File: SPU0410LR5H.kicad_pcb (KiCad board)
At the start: 2 copper layers, 23 x 12.5 mm, 17 parts, among them J1 Conn_01x04_Pin, U1 MCP6002-xSN, U2 SPU0410LR5H-QB

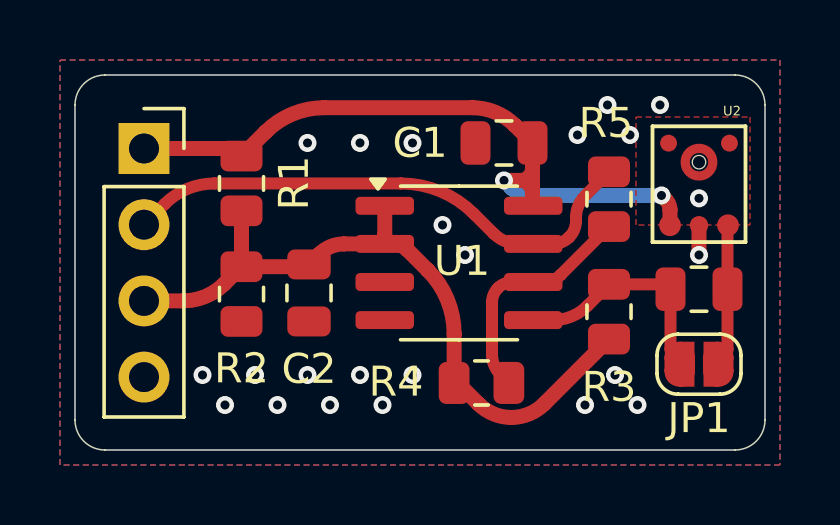
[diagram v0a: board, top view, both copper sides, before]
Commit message: update silkscreen
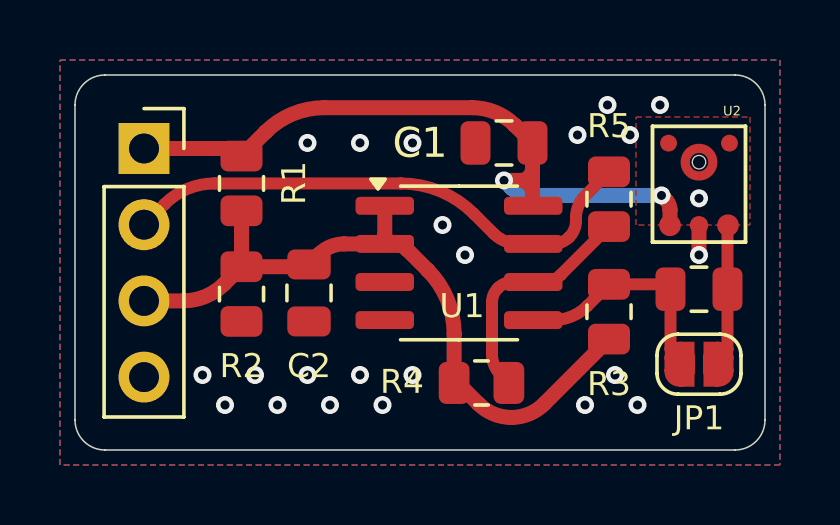
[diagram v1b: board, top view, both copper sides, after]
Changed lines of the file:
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@@
 			(outputformat 1)
 			(mirror no)
-			(drillshape 1)
+			(drillshape 0)
 			(scaleselection 1)
-			(outputdirectory "")
+			(outputdirectory "gerbers")
 		)
 	)
@@
 		(tags "resistor")
 		(property "Reference" "R2"
-			(at 2.48 0 180)
+			(at 2.397501 0 180)
 			(layer "F.SilkS")
 			(effects
 				(font
-					(size 1 1)
+					(size 0.8 0.8)
 					(thickness 0.15)
 				)
@@
 		(tags "capacitor")
 		(property "Reference" "C2"
-			(at -2.535 0 0)
+			(at -2.435001 0 0)
 			(layer "F.SilkS")
 			(effects
 				(font
-					(size 1 1)
+					(size 0.8 0.8)
 					(thickness 0.15)
 				)
@@
 			(effects
 				(font
-					(size 1 1)
+					(size 0.8 0.8)
 					(thickness 0.15)
 				)
@@
 		(tags "resistor")
 		(property "Reference" "R5"
-			(at 2.54 -0.1 180)
+			(at 2.439999 0 180)
 			(layer "F.SilkS")
 			(effects
 				(font
-					(size 1 1)
+					(size 0.8 0.8)
 					(thickness 0.15)
 				)
@@
 		(tags "resistor")
 		(property "Reference" "R3"
-			(at -2.51 0 180)
+			(at -2.410001 0 180)
 			(layer "F.SilkS")
 			(effects
 				(font
-					(size 1 1)
+					(size 0.8 0.8)
 					(thickness 0.15)
 				)
@@
 		(tags "SOIC SO")
 		(property "Reference" "U1"
-			(at 0.1 -0.065 0)
+			(at 0.1 1.435001 0)
 			(layer "F.SilkS")
 			(effects
 				(font
-					(size 1 1)
+					(size 0.8 0.8)
 					(thickness 0.15)
 				)
@@
 			(effects
 				(font
-					(size 1 1)
+					(size 0.8 0.8)
 					(thickness 0.15)
 				)
@@
 		(tags "resistor")
 		(property "Reference" "R4"
-			(at -2.85 -0.04 0)
+			(at -2.649999 -0.04 0)
 			(layer "F.SilkS")
 			(effects
 				(font
-					(size 1 1)
+					(size 0.8 0.8)
 					(thickness 0.15)
 				)
@@
 		)
 	)
-	(group ""
-		(members "0188a09c-7b3a-4e7d-b924-1a51db423fca" "01dd3f70-7b91-45b8-8625-1166b87dc310"
-			"06bd51c4-d7e4-4a8e-bd02-fb3527cab53b" "07391707-5658-49a0-982e-18ab20bf6a0b"
-			"0bc5ff85-6a44-442d-bb75-140a14e7ecda" "0ff94fb2-d96d-485c-af0e-3a3204c8d92e"
-			"1ec9dda9-f6cd-4c76-989f-f296964f100c" "1f687e2a-3e9e-4f34-a8db-d5ed2ac7a032"
-			"226cf68c-6454-4a30-9ba6-72346a1b9594" "25902495-e8ad-4b9f-86e3-a440dd0bdc7d"
-			"26ac06f0-dbe7-4740-aebd-eb0e6bc05efa" "275047c7-ff20-4189-a30a-68d29308208a"
-			"281790e6-05f2-4878-8b64-6fee776a12cb" "28fe2402-5fae-490c-bdbd-93c1f81c649b"
-			"290768fa-1b14-464a-bce2-6f304fa074e5" "2928b064-24c8-4e05-8e86-d27e9670b574"
-			"2c890f45-1aa6-43ea-858f-020b7474a7ad" "2d97d7dd-1ab0-400c-85dc-c5eb09f0a0d2"
-			"31988b26-4ece-4f10-8980-1628ae3e36a1" "34e5e205-2e19-4c54-a946-d463a5158fb5"
-			"38536011-8b32-45a5-83ff-be7c7b0e5ecb" "3ac29b50-73a1-4827-a6ff-f9a69546019e"
-			"3d85da51-d6fb-4ea7-8ef1-b61cd9b7c2b3" "3eb430aa-e8b6-4546-af6d-e0d8b82b6ff7"
-			"3fad04cc-d1bc-4f39-8a0b-cc47cc63b91f" "40c28612-1eb8-4802-83d9-aa82f6037516"
-			"451b7ac5-6ed7-4ea0-aaf9-2d634aa81f74" "45b2b29f-4285-458d-b20b-41dfb74df641"
-			"484eba7e-3cbf-4f44-a601-ec708db228b8" "4ae74bf4-ef4c-410d-938e-ae50d2f7056a"
-			"4f9280a8-f1f9-4f28-a080-208dfc8adc60" "4fffb4b6-cc3e-451e-baee-728d49727d52"
-			"500d8281-30fe-4550-9e20-595132cb9a63" "53558727-af01-477e-afcb-dd3c699c5dc9"
-			"54dd1572-65bf-4502-a9af-95ec9dd3487a" "5ab70692-9651-4b40-8feb-3e774b2a4d9e"
-			"5b4af646-af64-46e4-9a0a-a9be29fef6c4" "5ce2e46c-c89c-4e5c-9d56-2ee28f6d0800"
-			"5e869954-1c73-401f-8f3c-b8bd25f15bb9" "5f083619-73df-47be-8548-d462a89ac208"
-			"6b30f90f-69a1-46a8-9d01-0f73f3134ca8" "6ca4cad8-7fd5-4171-ab1b-1ca6c5714486"
-			"6e9d763a-9b92-4978-a805-58f769d68813" "6f990783-8769-41d8-8786-cd0714114efd"
-			"747bbb79-58cd-41c4-8c08-27f0f3b7294e" "77d47272-09c1-49cc-ba08-75a3beb473f9"
-			"7a04422b-64c7-4421-a0ad-a7a532d65c40" "7a04500e-16cf-419e-835f-9f64a12b3d31"
-			"7e681bcf-2422-4c44-b800-77a06061e357" "81ebadf8-634c-4840-8f12-62b452058382"
-			"8319fdc5-94b3-4b18-8166-f85d2afd45cb" "84249f85-0442-4b1c-b5a3-acf17100d5b6"
-			"8a965b55-07a8-4b29-8d3a-82c0e194f63f" "8d8eb7bd-2d64-4287-b43f-941243b7038b"
-			"8e299b2a-d96b-4ff3-9ff2-0591982ed3d9" "8fd1f4fa-7689-459e-b902-d1e822ce0e9a"
-			"92f9ee2d-21be-46ea-b105-498461660311" "93f48a04-185d-46ff-8f33-199d65f33eb7"
-			"99bf1a58-f5ec-4ba3-aabb-31ea3ab382d5" "9a373ff2-7db0-40b8-bcca-8081f7042301"
-			"9b661790-1dfc-474a-9a53-6a754c2a0338" "9d43cc62-dc1c-4f33-92d8-1dc76437202f"
-			"a01ee861-9f16-4ba8-939e-6af2d37722e4" "a04ace39-668a-4772-933c-36917ae04930"
-			"a1acf204-7a94-446d-b77b-331efab4e0ba" "a23125df-4d3c-4e88-a3f7-93370b916c51"
-			"a331b85b-ed78-4651-894a-459fca82e0d7" "af28cf7a-1597-403e-8f9e-988bb2525df6"
-			"b0552b33-d5fb-4fdb-9a3a-185486a27ea9" "b0743439-3831-4326-9f77-ae5cffe5ea93"
-			"b0ade9f1-98ad-43f8-8508-38b9b8618af4" "b42cc91b-2c18-4de8-9c68-0843cb291165"
-			"b732ec15-4b6d-4506-883e-5962f745083d" "c042527f-e3c8-4599-92ad-5e28a872d0d8"
-			"c1b32af8-fd6f-45ca-9744-3673f4e6fd27" "c4366db1-6edd-4c54-8f46-cb0d607410d2"
-			"cb11fbe2-cc76-47ac-a88a-debfa6c5511e" "cc8dcb07-23a2-456e-b957-9663ea418fcc"
-			"cd3a56aa-e1d3-4229-a8a6-06708be20cf4" "cf24944f-74dc-4627-8a33-ae9e81b28a9a"
-			"d084d465-c392-454f-9810-497c2369e9b2" "d39097b8-9785-4fd0-b033-d6c83c165e6d"
-			"d554d984-5711-4919-b90d-6566b3ffdb50" "d56ac40f-429d-48ab-8ed3-75fe905959bc"
-			"d775586a-54c2-4df6-88b5-845dd0788a2f" "dc741dec-69a6-4fd9-aa29-3f9565c74df9"
-			"dcaf0d53-63eb-41b9-abae-ad711014ed1c" "e18b405e-7d84-4dfb-82ba-19311d630cff"
-			"e2e25fa2-58ac-42c8-bf8f-946a5a8da1d0" "e62e2b33-a34e-4bb7-95a0-03b061a0c213"
-			"eba3c1a7-e4e5-4cf1-8f92-8c625f7a8d24" "f625b1d1-029b-4090-a4c8-03f7544a954d"
-			"f68cd0ce-a217-41d2-996c-479d4bc87243" "f88abe03-73d9-4d0f-b8ae-72287abc74d4"
-			"fbc10ced-c5e1-4969-ae70-bb2f55cea9cc" "fce6fc82-a280-40ae-ab8d-1946d4b50dd0"
-		)
-	)
